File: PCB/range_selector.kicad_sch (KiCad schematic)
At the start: 23 parts, among them U106 74HC00, U201 74HC193, U202 74HC139, U203 74HC14

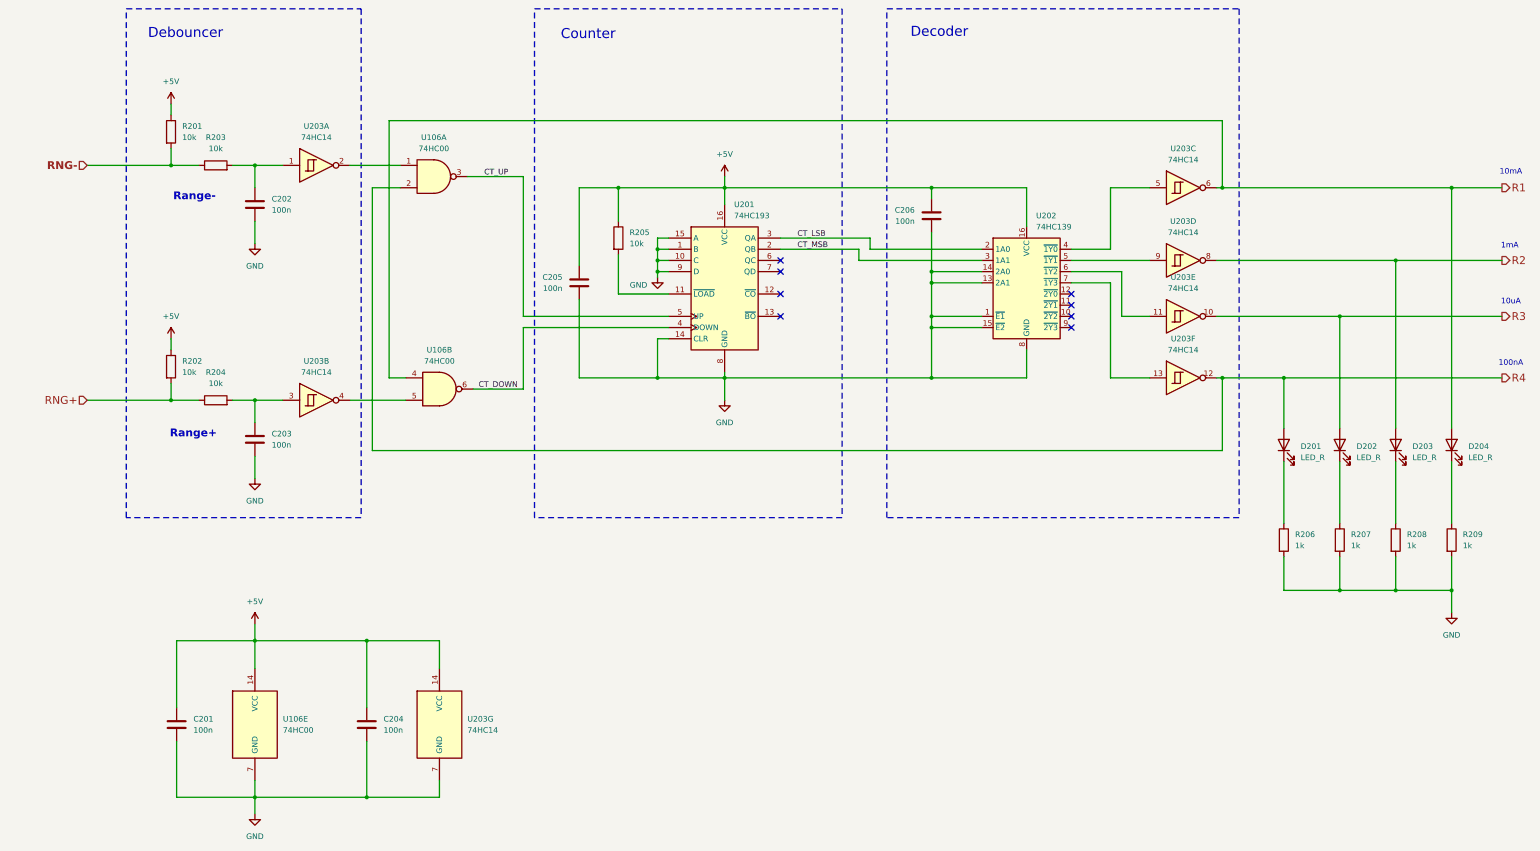
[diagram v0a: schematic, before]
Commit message: start of layout
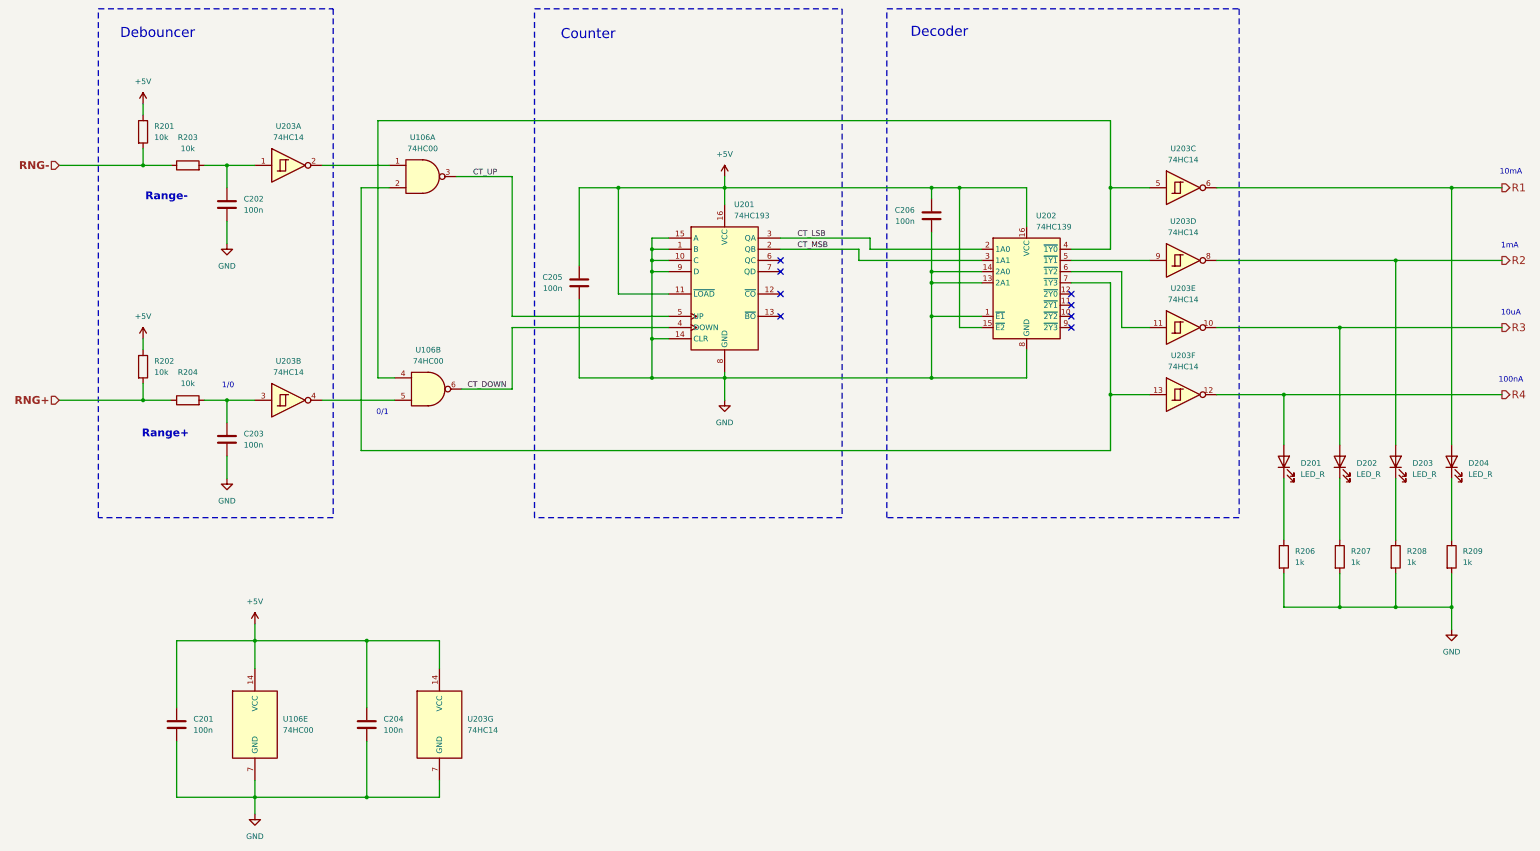
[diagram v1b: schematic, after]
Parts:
- removed R205: 10k, Resistor_SMD:R_0603_1608Metric, symbol Device:R
- D201, D202, D203, D204: footprint LED_SMD:LED_0603_1608Metric -> LED_THT:LED_D3.0mm
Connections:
- net +5V: now also U201.11 (~{LOAD}), U202.15 (~{E2})
- net GND: no longer U202.15 (~{E2})
- net R1: no longer U106.4
- net R4: no longer U106.2
- net at U202.4 (~{1Y0}), U203.5: now also U106.4
- net at U202.7 (~{1Y3}), U203.13: now also U106.2
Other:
- note added: "0/1"
- note added: "1/0"
- moved on the sheet: C202, C203, D201, D202, D203, D204, R201, R202, R203, R204, R206, R207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
